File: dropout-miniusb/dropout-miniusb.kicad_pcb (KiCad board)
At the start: 2 copper layers, 75 x 94.1 mm, 47 parts, among them SW1 Rotary_Encoder_Switch, SW2 SW_Push, U1 ProMicro

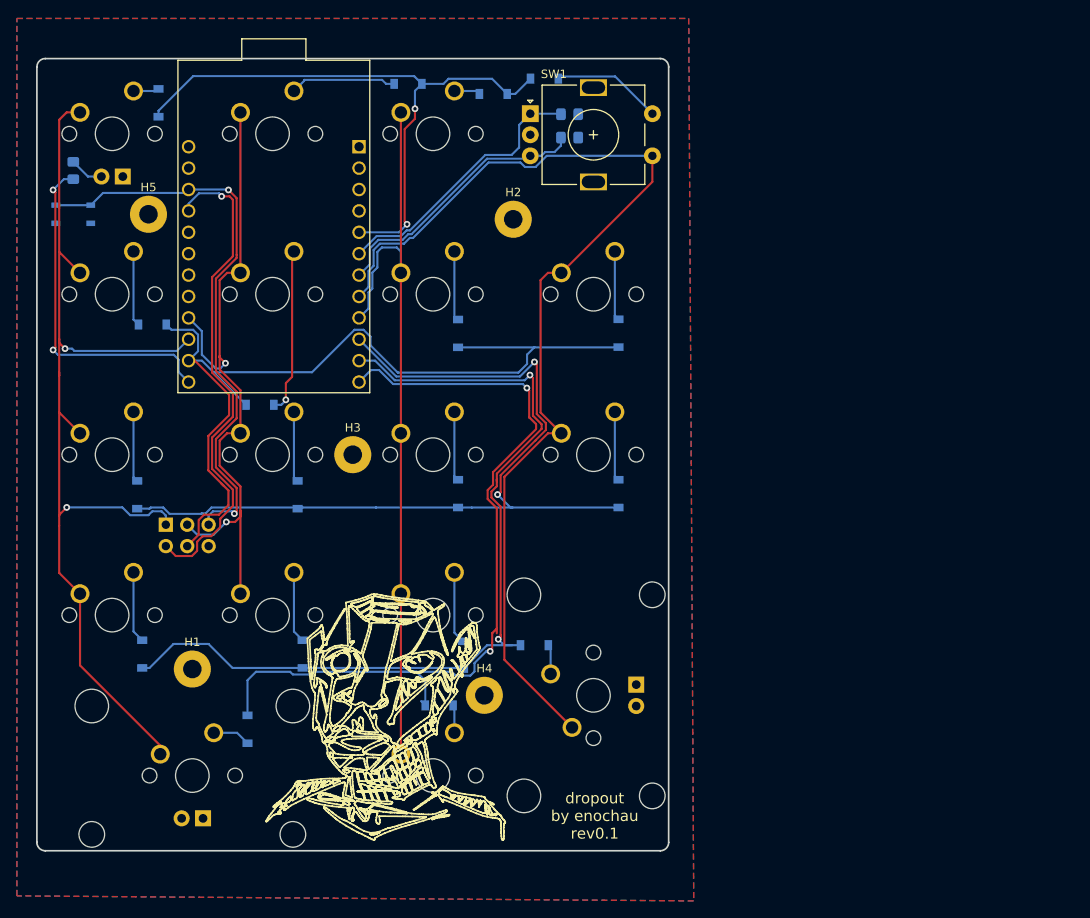
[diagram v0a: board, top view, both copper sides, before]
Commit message: cleanup
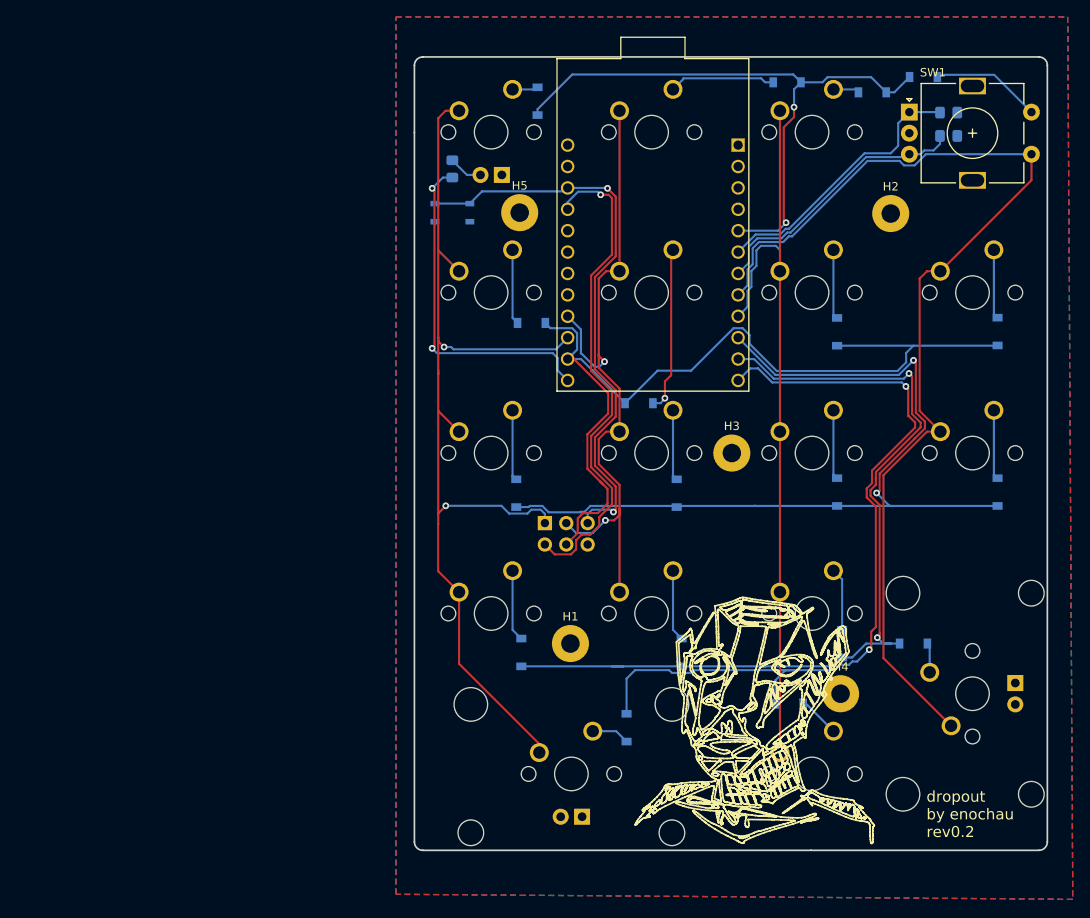
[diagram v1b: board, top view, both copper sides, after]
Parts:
- moved D13 45.0 mm to (188.3, 120.2)
- moved D1 45.0 mm to (152.2, 55.8)
- moved J-ISP1 45.0 mm to (153.0, 105.9)
- moved C1 45.0 mm to (201.0, 59.9)
- moved C2 45.0 mm to (201.0, 57.2)
- moved D11 45.0 mm to (187.7, 83.2)
- moved D12 45.0 mm to (187.7, 102.2)
- moved D15 45.0 mm to (198.0, 52.9)
- moved D16 45.0 mm to (206.8, 83.2)
- moved D17 45.0 mm to (206.8, 102.2)
- moved D18 45.0 mm to (196.8, 120.2)
- moved D2 45.0 mm to (151.4, 82.1)
- moved D3 45.0 mm to (149.6, 102.3)
- moved D4 45.0 mm to (150.2, 121.3)
- moved D5 45.0 mm to (162.7, 130.2)
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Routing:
- net Net-(D14-Pad2): track 3.32 -> 5.64 mm
- net ROW1: track 110.7 -> 108.5 mm
- net ROW4: track 99.5 -> 97.8 mm
- net Net-(D13-Pad2): track 8.62 -> 7.43 mm
- net ROW3: track 107.5 -> 106.4 mm
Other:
- board size 75 x 94.1 mm -> 75.1 x 94.2 mm
- board text added: "dropout by enochau rev0.2"
- board text removed: "dropout by enochau rev0.1"
